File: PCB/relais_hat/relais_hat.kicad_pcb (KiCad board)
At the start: 4 copper layers, 85 x 56 mm, 61 parts, among them J1 Conn_01x03, J10 Conn_01x02, J11 Conn_01x02, J12 Conn_01x03, J13 DB9_Female, J14 Conn_01x02, J15 Conn_01x02, J16 Conn_01x02, J17 Conn_01x02, J18 Conn_01x02, J2 Conn_01x03, J3 Conn_02x04_Odd_Even, J4 Screw_Terminal_01x02, J5 Screw_Terminal_01x02, J6 Screw_Terminal_01x02, J7 Screw_Terminal_01x02, J8 Conn_01x02, J9 Conn_01x02, K1 RELAY-HLS8L-DC3V-S-C(5P-19X15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, K2 RELAY-HLS8L-DC3V-S-C(5P-19X15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, K3 RELAY-HLS8L-DC3V-S-C(5P-19X15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, K4 RELAY-HLS8L-DC3V-S-C(5P-19X15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, P1 Conn_02x20_Odd_Even, Q1 S8050, Q2 S8050, Q3 S8050, Q4 S8050, U1 XC6206P302MR-G, U2 XC6206P302MR-G, U3 XC6206P302MR-G, U4 XC6206P302MR-G

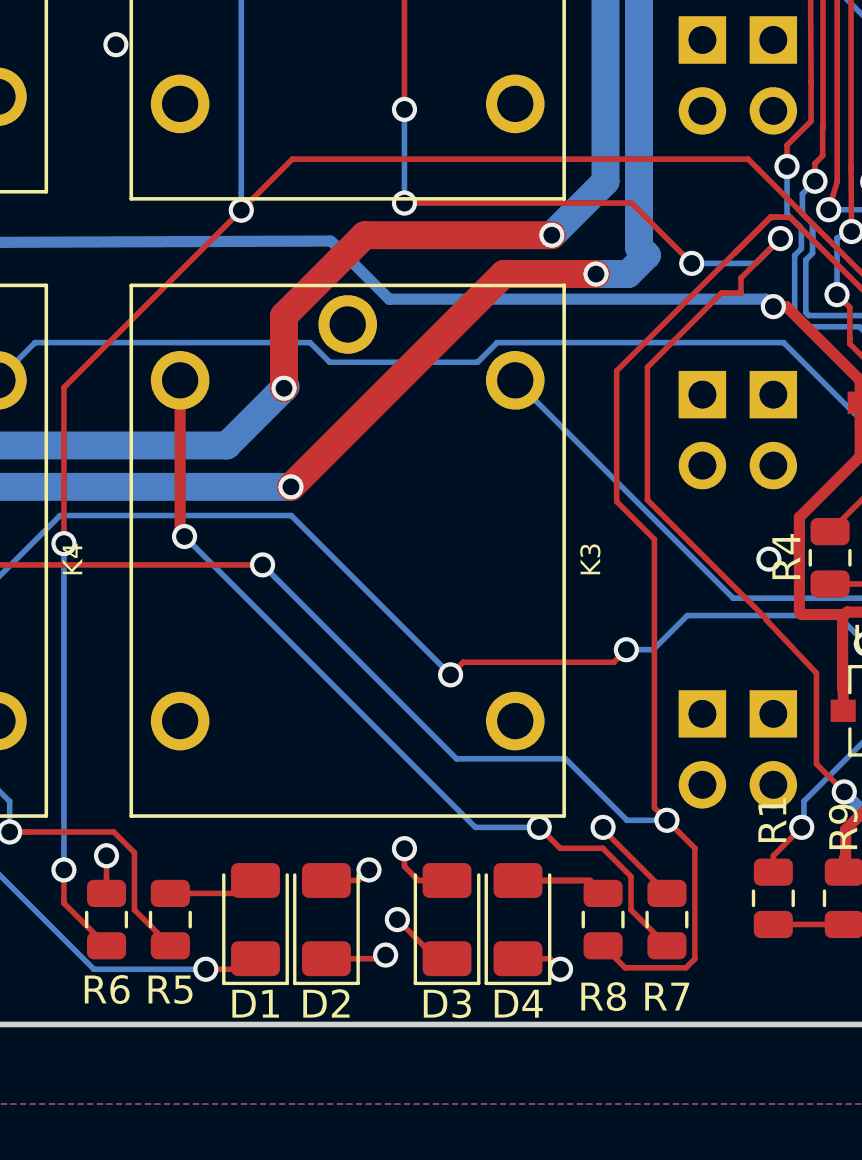
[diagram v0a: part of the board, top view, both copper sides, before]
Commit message: ajust all board
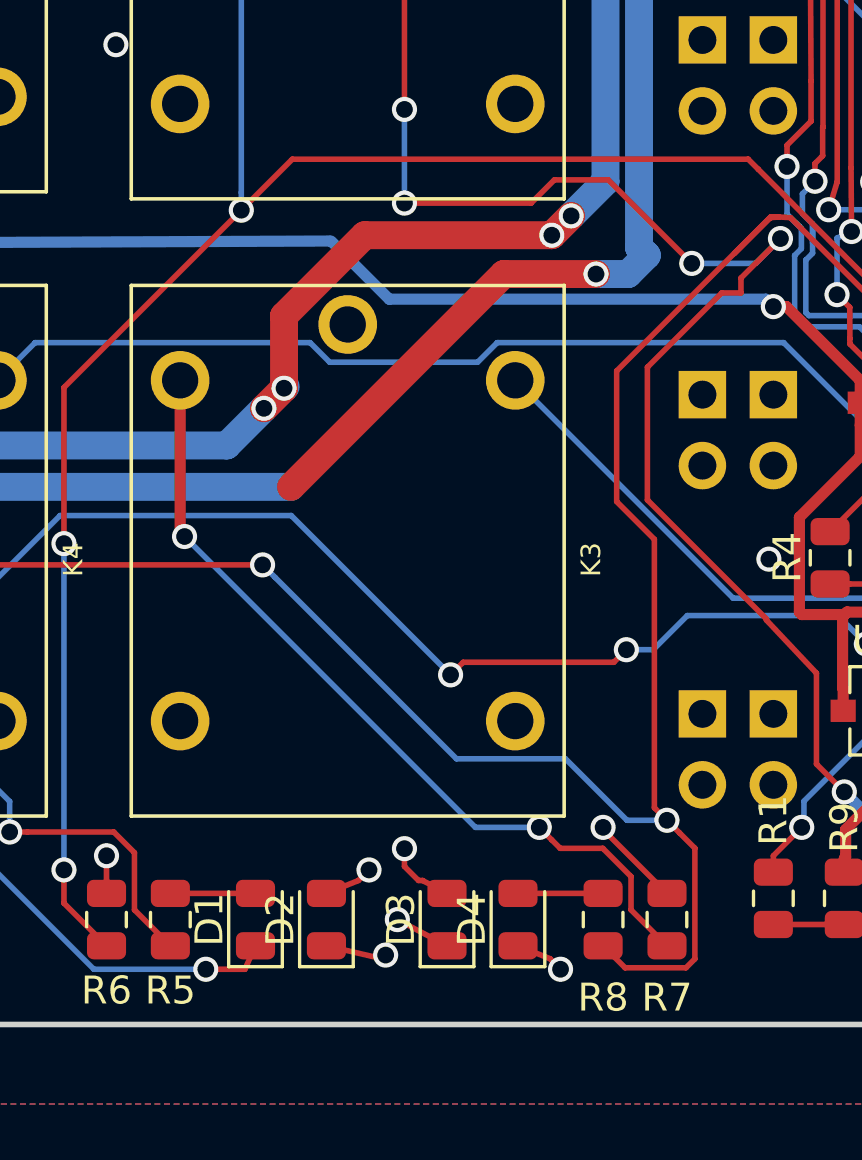
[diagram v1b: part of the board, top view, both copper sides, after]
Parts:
- D1, D2, D3, D4: footprint LED_SMD:LED_1206_3216Metric -> LED_SMD:LED_0805_2012Metric
- MK1, MK2, MK3, MK4: value M2.5 -> M3
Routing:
- net Net-(D4-Pad2): track 6.08 -> 3.05 mm
- net Net-(D2-Pad1): track 105.7 -> 106.5 mm
- net +12V: vias 2 -> 4
- net GND: vias 11 -> 10
